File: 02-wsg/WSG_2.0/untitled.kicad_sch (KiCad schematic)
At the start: 28 parts, among them IC1 W25N04KVZEIR, IC5 AP2120N-3.3TRG1, IC8 SPX3819S-L_TR, J1 USB4110-GF-A, J4 Conn_01x02, U1 BQ21040DBVR

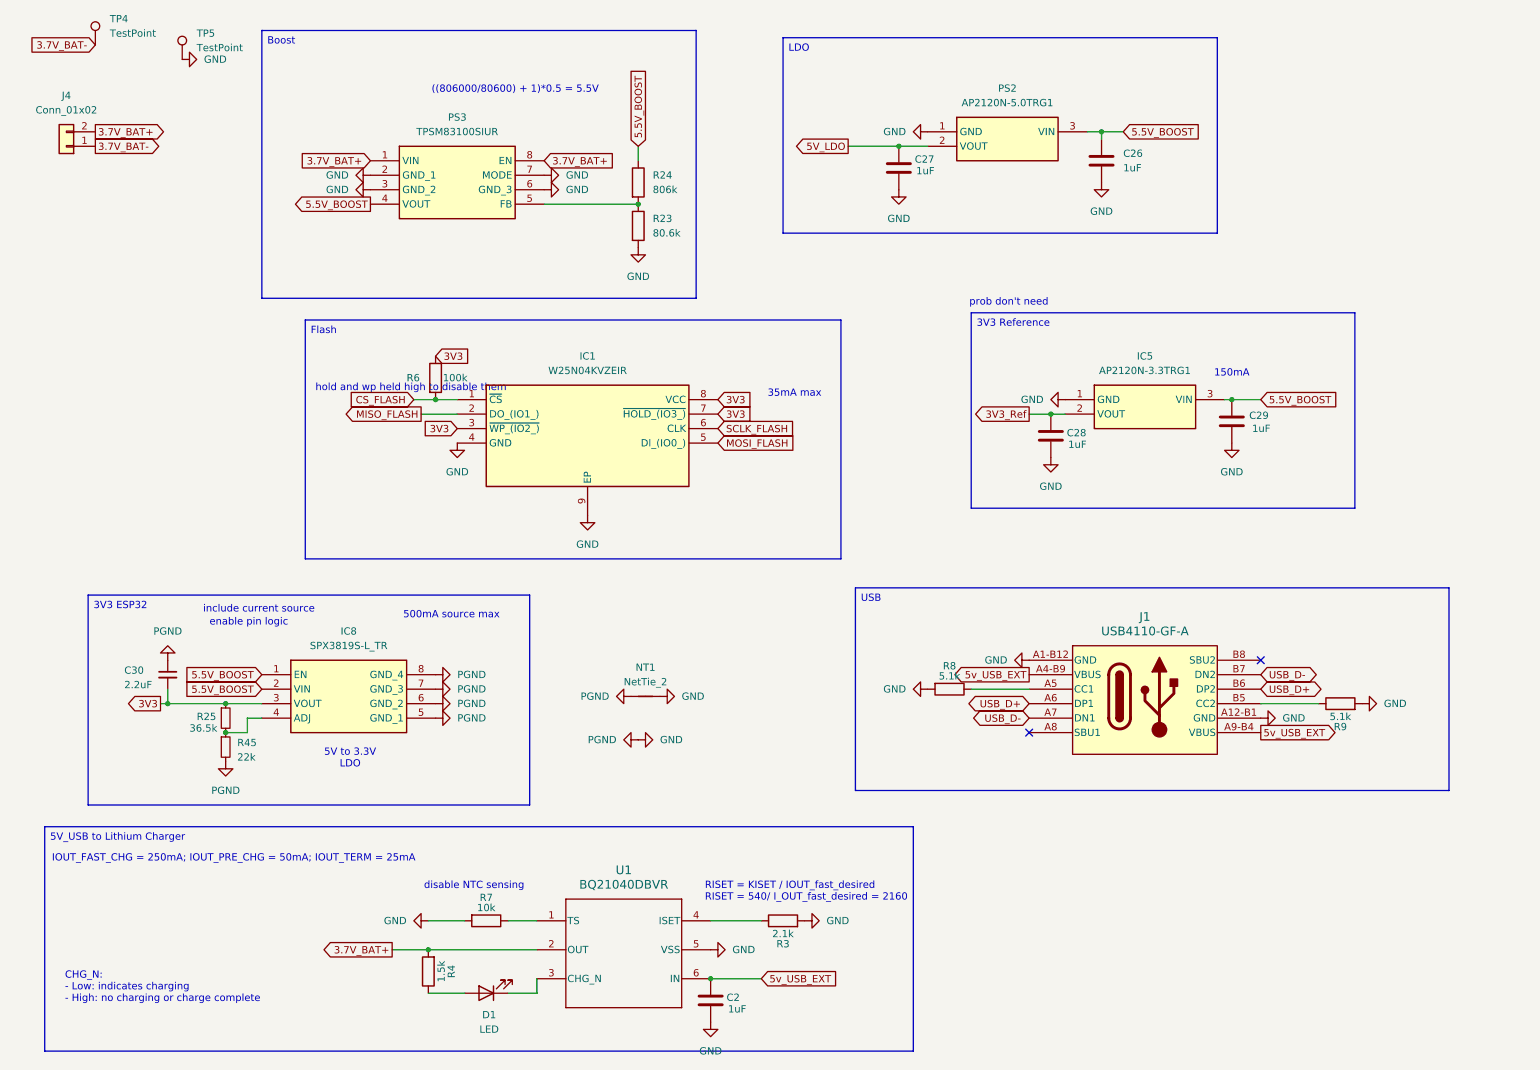
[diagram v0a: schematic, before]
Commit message: layout and schematic updates
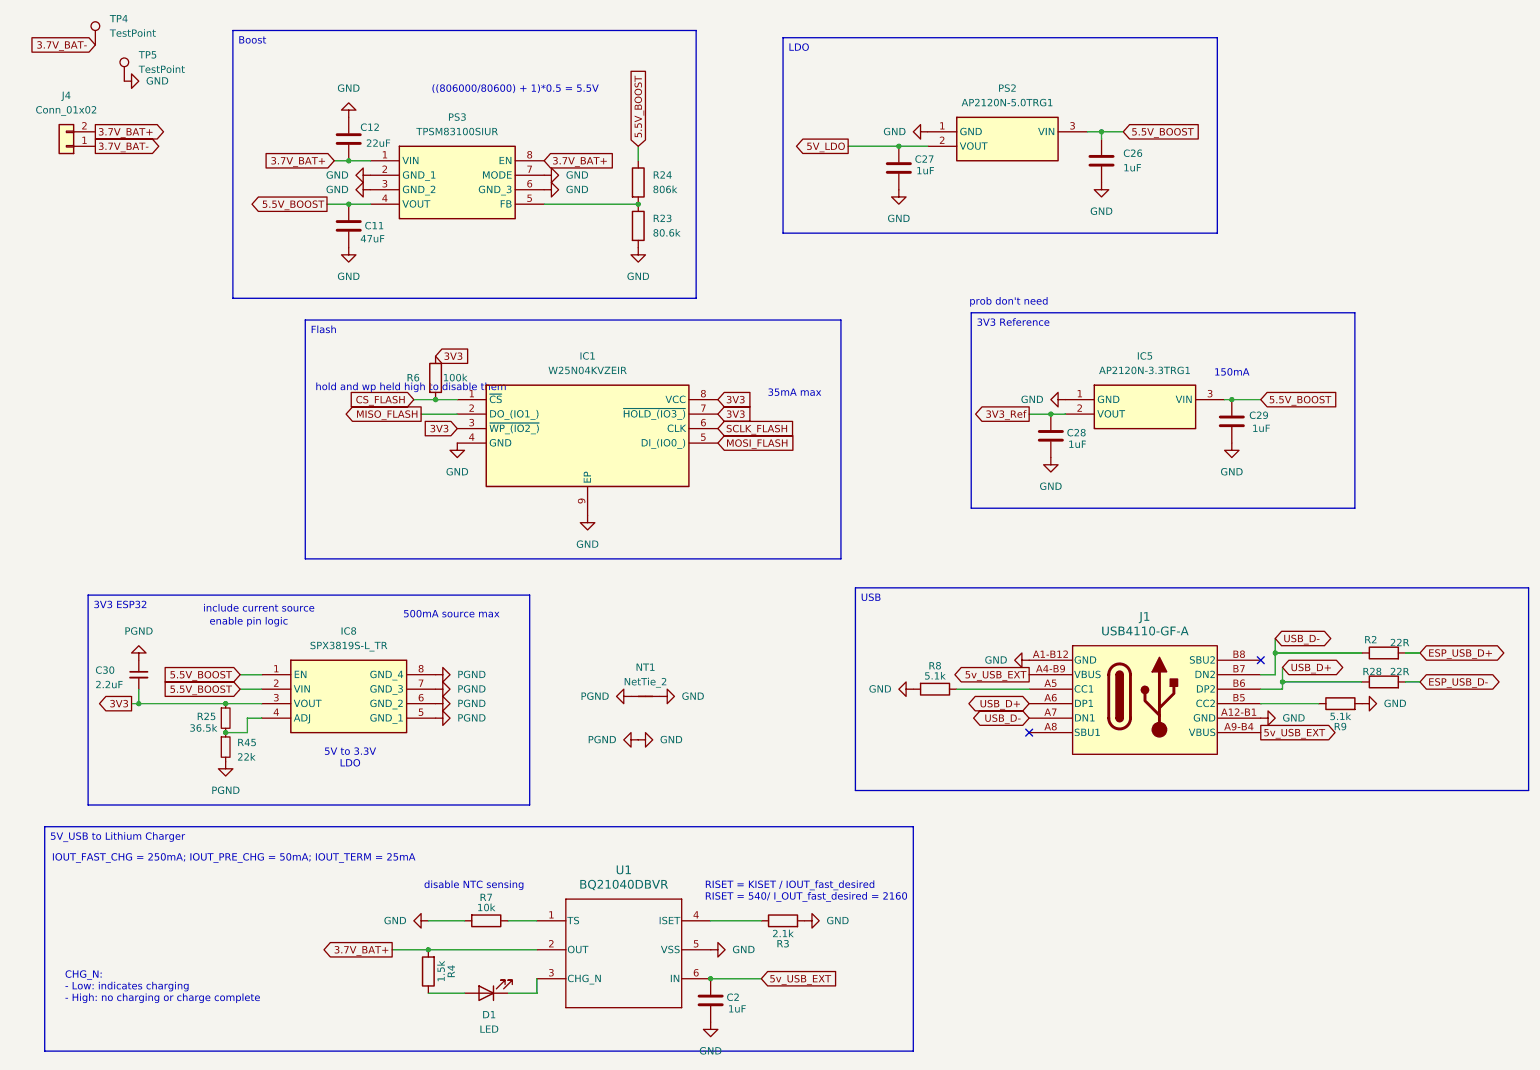
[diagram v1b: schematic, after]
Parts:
- added C11: 47uF, Capacitor_SMD:C_0402_1005Metric, symbol Device:C
- added C12: 22uF, Capacitor_SMD:C_0402_1005Metric, symbol Device:C
- added R2, R28: 22R, Resistor_SMD:R_0402_1005Metric, symbol Device:R
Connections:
- net 3.7V_BAT+: now also C12.2
- net 5.5V_BOOST: now also C11.1
- net GND: now also C11.2, C12.1
- net USB_D+: now also R28.1
- net USB_D-: now also R2.1
- new net ESP_USB_D+: R2.2
- new net ESP_USB_D-: R28.2
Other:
- moved on the sheet: C30, R8, TP5
